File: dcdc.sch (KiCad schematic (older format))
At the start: 14 parts, among them IC2 OKR-T_6-W12-C, J2 Header_2x6_2.54mm

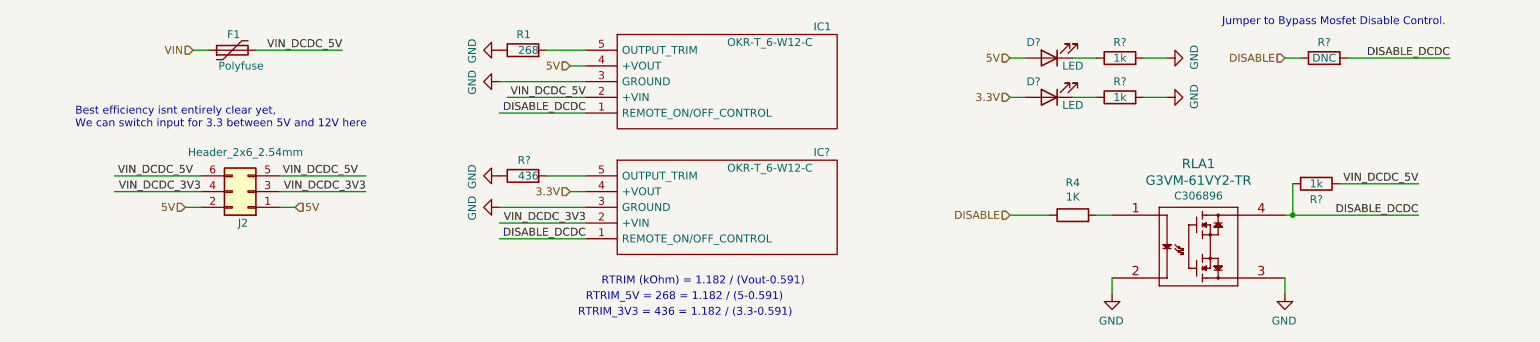
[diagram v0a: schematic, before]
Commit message: Organized pi.sch document.
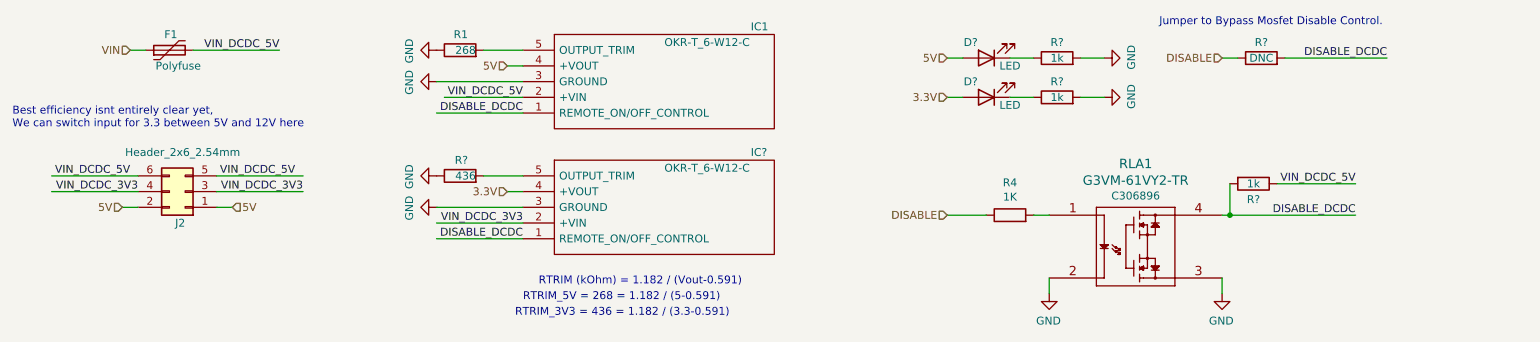
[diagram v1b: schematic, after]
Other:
- moved on the sheet: D?, F1, IC1, IC?, J2, R1, R4, R?, RLA1
